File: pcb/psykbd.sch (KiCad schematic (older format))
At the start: 16 parts, among them SW1 SW_PUSH, U1 ATmega32U4-AU, Y1 16MHz

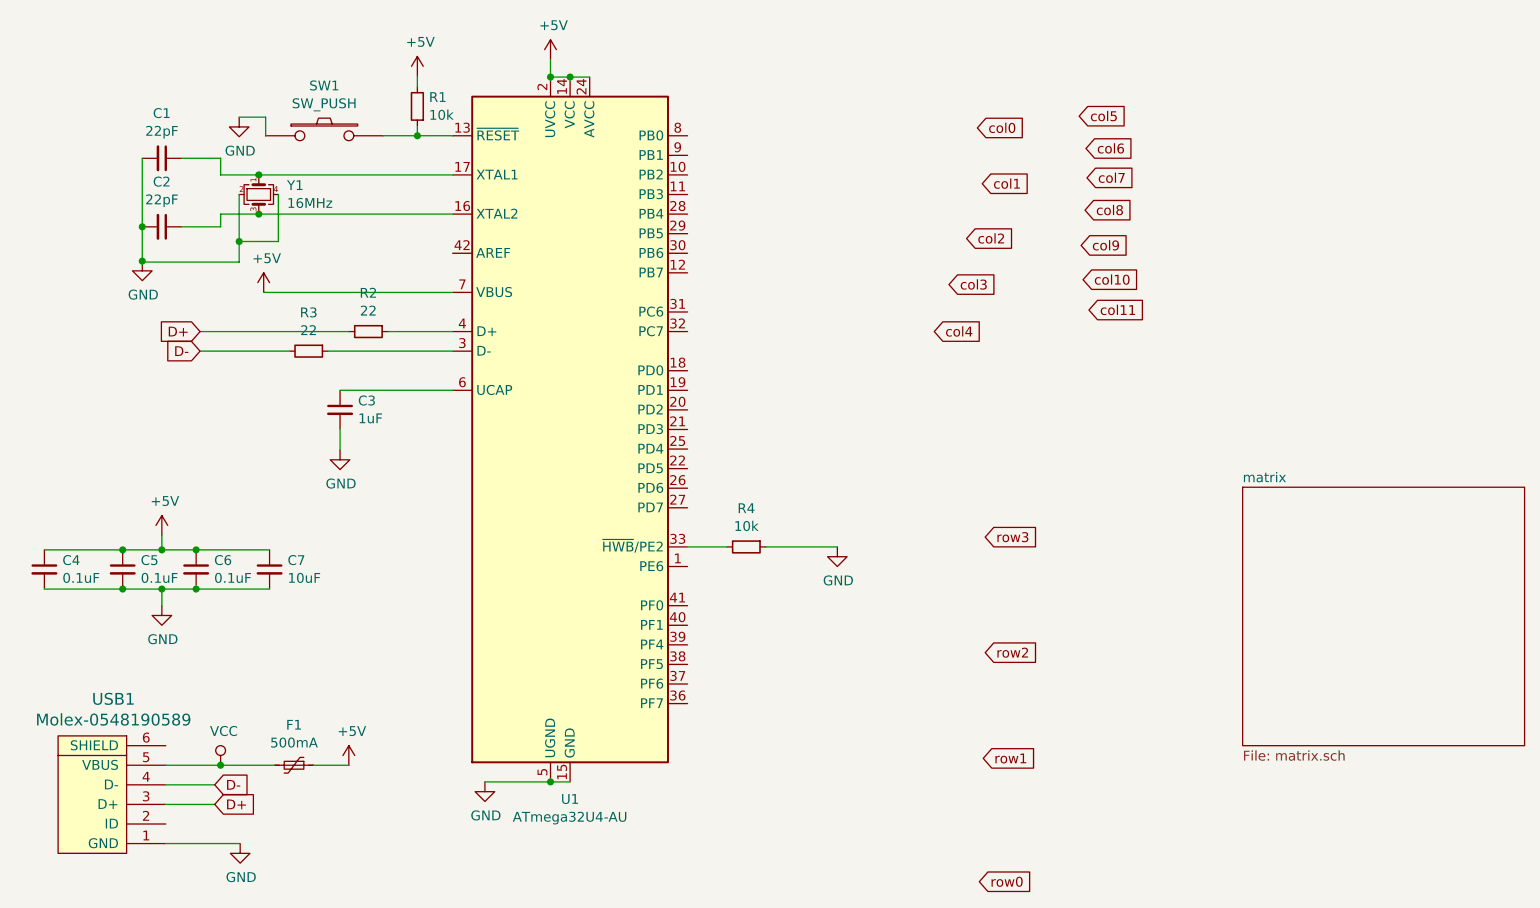
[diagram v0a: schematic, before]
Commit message: Routing
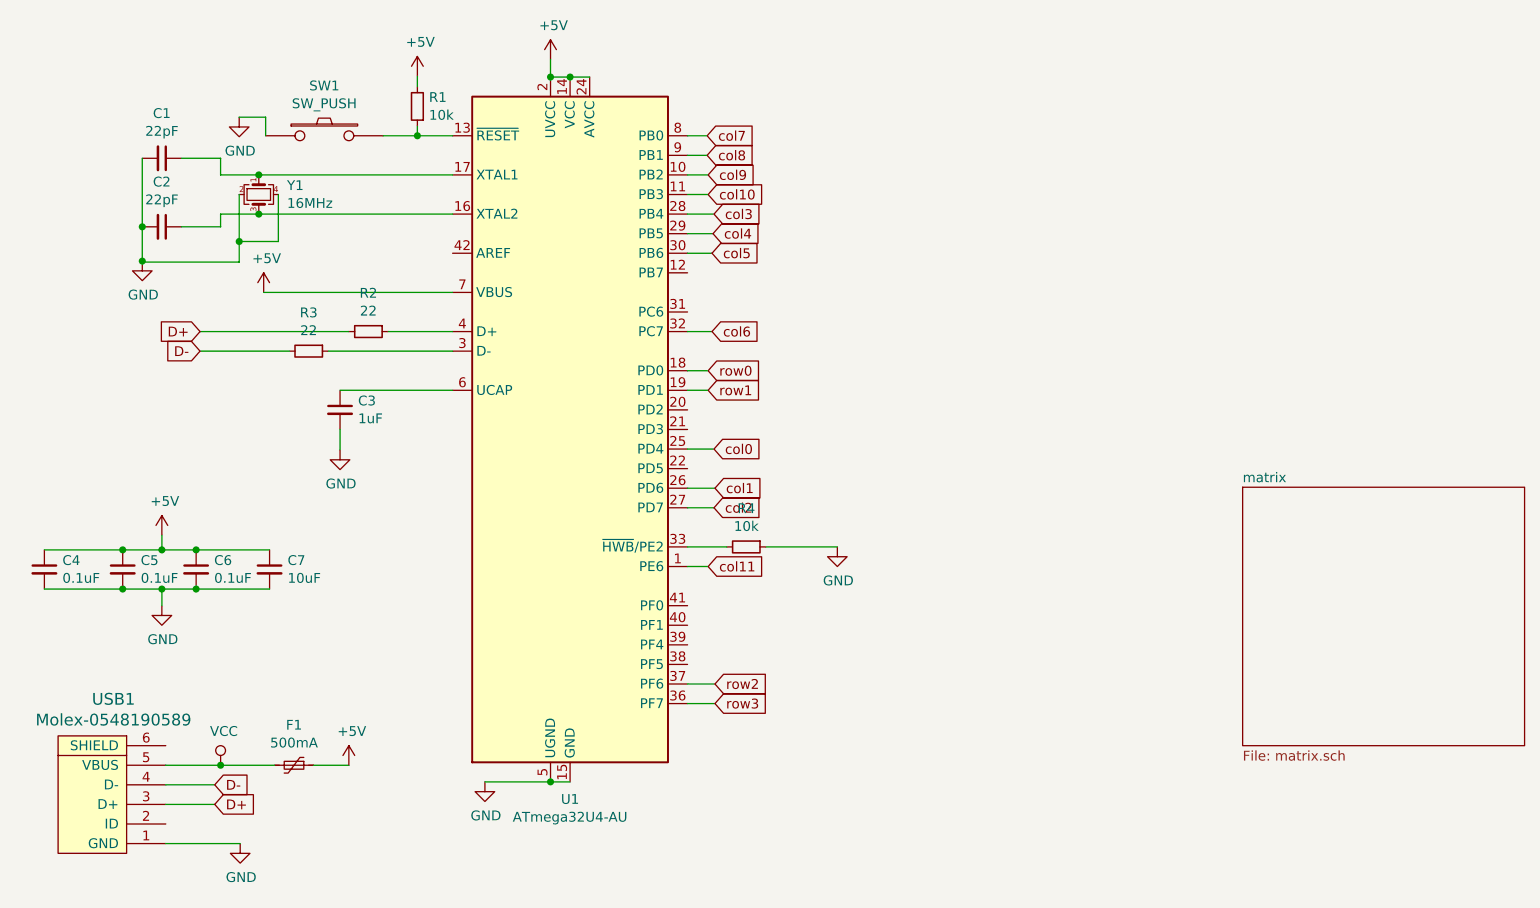
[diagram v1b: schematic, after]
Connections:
- net col0: now also U1.25 (PD4)
- net col1: now also U1.26 (PD6)
- net col10: now also U1.11 (PB3)
- net col11: now also U1.1 (PE6)
- net col2: now also U1.27 (PD7)
- net col3: now also U1.28 (PB4)
- net col4: now also U1.29 (PB5)
- net col5: now also U1.30 (PB6)
- net col6: now also U1.32 (PC7)
- net col7: now also U1.8 (PB0)
- net col8: now also U1.9 (PB1)
- net col9: now also U1.10 (PB2)
- net row0: now also U1.18 (PD0)
- net row1: now also U1.19 (PD1)
- net row2: now also U1.37 (PF6)
- net row3: now also U1.36 (PF7)
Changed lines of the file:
@@
 Wire Wire Line
 	3425 990  3425 900
-Connection ~ 3425 4590
-Connection ~ 3525 990
-Connection ~ 3425 990
-Wire Wire Line
-	3625 990  3525 990
-Wire Wire Line
-	3525 4590 3425 4590
-Wire Wire Line
-	3525 990  3425 990
 $Comp
 L power:GND #PWR0102
@@
 $EndComp
 $Comp
-L MCU_Microchip_ATmega:ATmega32U4-AU U1
-U 1 1 5E0DFF6A
-P 3525 2790
-F 0 "U1" H 3525 901 50  0000 C CNN
-F 1 "ATmega32U4-AU" H 3525 810 50  0000 C CNN
-F 2 "Package_QFP:TQFP-44_10x10mm_P0.8mm" H 3525 2790 50  0001 C CIN
-F 3 "http://ww1.microchip.com/downloads/en/DeviceDoc/Atmel-7766-8-bit-AVR-ATmega16U4-32U4_Datasheet.pdf" H 3525 2790 50  0001 C CNN
-	1    3525 2790
-	1    0    0    -1
-$EndComp
-Wire Wire Line
-	3090 4590 3425 4590
-$Comp
 L Device:R_Small R4
 U 1 1 5E0EAE60
@@
 	1    0    0    -1
 $EndComp
-Wire Wire Line
-	4125 3390 4325 3390
 Wire Wire Line
 	4525 3390 4890 3390
@@
 F1 "matrix.sch" 50
 $EndSheet
-Text GLabel 5605 1250 2    50   Input ~ 0
+Text GLabel 4260 3190 2    50   Input ~ 0
+col2
+Text GLabel 4260 1690 2    50   Input ~ 0
+col3
+Text GLabel 4255 1790 2    50   Input ~ 0
+col4
+Text GLabel 4250 1890 2    50   Input ~ 0
+col5
+Text GLabel 4250 2290 2    50   Input ~ 0
+col6
+Text GLabel 4225 1290 2    50   Input ~ 0
+col7
+Text GLabel 4225 1390 2    50   Input ~ 0
+col8
+Text GLabel 4230 1490 2    50   Input ~ 0
+col9
+Text GLabel 4230 1590 2    50   Input ~ 0
+col10
+Text GLabel 4265 4190 2    50   Input ~ 0
+row3
+Text GLabel 4265 4090 2    50   Input ~ 0
+row2
+Text GLabel 4230 2590 2    50   Input ~ 0
+row1
+Text GLabel 4230 2490 2    50   Input ~ 0
+row0
+Wire Wire Line
+	4125 1390 4225 1390
+Wire Wire Line
+	4125 1490 4230 1490
+Wire Wire Line
+	4125 1590 4230 1590
+Text GLabel 4260 2890 2    50   Input ~ 0
 col0
-Text GLabel 5630 1535 2    50   Input ~ 0
+Connection ~ 3425 4590
+Connection ~ 3525 990
+Connection ~ 3425 990
+Wire Wire Line
+	3625 990  3525 990
+Wire Wire Line
+	3525 990  3425 990
+Wire Wire Line
+	3525 4590 3425 4590
+Wire Wire Line
+	3090 4590 3425 4590
+Wire Wire Line
+	4265 4190 4125 4190
+Wire Wire Line
+	4265 4090 4125 4090
+Wire Wire Line
+	4125 3390 4325 3390
+Wire Wire Line
+	4125 2890 4260 2890
+Wire Wire Line
+	4125 2590 4230 2590
+Wire Wire Line
+	4230 2490 4125 2490
+Wire Wire Line
+	4250 2290 4125 2290
+Wire Wire Line
+	4125 1890 4250 1890
+Wire Wire Line
+	4125 1790 4255 1790
+Wire Wire Line
+	4125 1690 4260 1690
+Wire Wire Line
+	4260 3190 4125 3190
+$Comp
+L MCU_Microchip_ATmega:ATmega32U4-AU U1
+U 1 1 5E0DFF6A
+P 3525 2790
+F 0 "U1" H 3525 901 50  0000 C CNN
+F 1 "ATmega32U4-AU" H 3525 810 50  0000 C CNN
+F 2 "Package_QFP:TQFP-44_10x10mm_P0.8mm" H 3525 2790 50  0001 C CIN
+F 3 "http://ww1.microchip.com/downloads/en/DeviceDoc/Atmel-7766-8-bit-AVR-ATmega16U4-32U4_Datasheet.pdf" H 3525 2790 50  0001 C CNN
+	1    3525 2790
+	1    0    0    -1
+$EndComp
+Text GLabel 4265 3090 2    50   Input ~ 0
 col1
-Text GLabel 5550 1815 2    50   Input ~ 0
-col2
-Text GLabel 5460 2050 2    50   Input ~ 0
-col3
-Text GLabel 5385 2290 2    50   Input ~ 0
-col4
-Text GLabel 6125 1190 2    50   Input ~ 0
-col5
-Text GLabel 6160 1355 2    50   Input ~ 0
-col6
-Text GLabel 6165 1505 2    50   Input ~ 0
-col7
-Text GLabel 6155 1670 2    50   Input ~ 0
-col8
-Text GLabel 6135 1850 2    50   Input ~ 0
-col9
-Text GLabel 6145 2025 2    50   Input ~ 0
-col10
-Text GLabel 6175 2180 2    50   Input ~ 0
+Wire Wire Line
+	4265 3090 4125 3090
+Wire Wire Line
+	4225 1290 4125 1290
+Wire Wire Line
+	4125 3490 4230 3490
+Text GLabel 4230 3490 2    50   Input ~ 0
 col11
-Text GLabel 5645 3340 2    50   Input ~ 0
-row3
-Text GLabel 5645 3930 2    50   Input ~ 0
-row2
-Text GLabel 5635 4470 2    50   Input ~ 0
-row1
-Text GLabel 5615 5100 2    50   Input ~ 0
-row0
 $EndSCHEMATC
